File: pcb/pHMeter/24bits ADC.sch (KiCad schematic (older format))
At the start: 9 parts, among them J8 SJ, U6 HX711

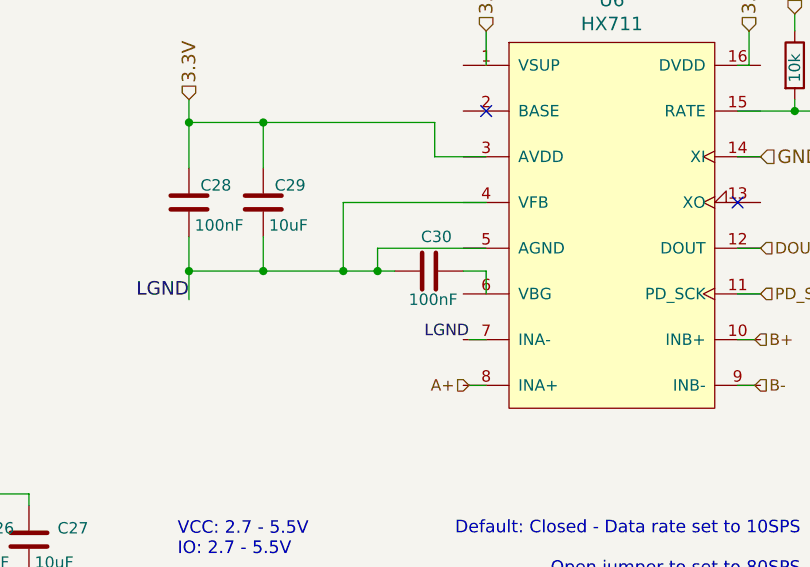
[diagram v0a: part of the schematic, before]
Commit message: Update pHMeter pcb
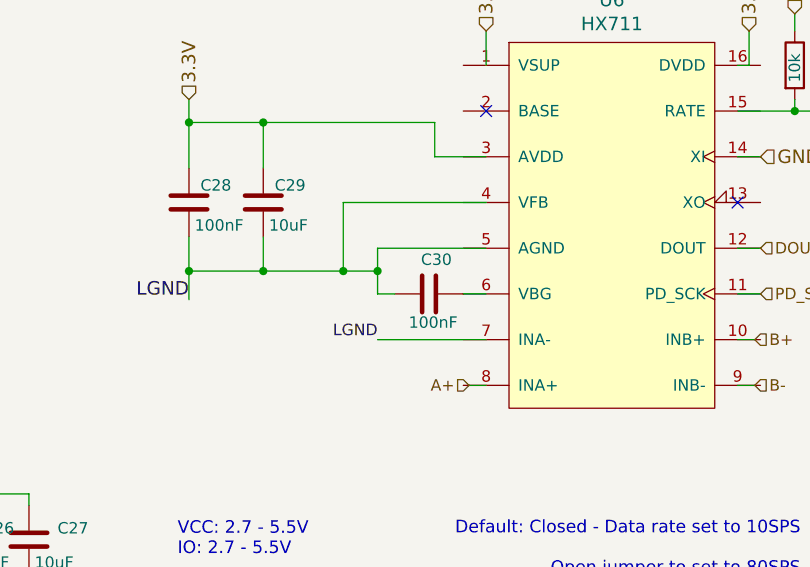
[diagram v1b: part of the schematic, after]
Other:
- moved on the sheet: C30
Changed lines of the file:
@@
 	3550 4600 3550 4700
-$Comp
-L Device:C C30
-U 1 1 5E3C27FC
-P 5875 3700
-F 0 "C30" V 6025 3600 50  0000 L CNN
-F 1 "100nF" V 5750 3575 50  0000 L CNN
-F 2 "Capacitor_SMD:C_0805_2012Metric_Pad1.15x1.40mm_HandSolder" H 5913 3550 50  0001 C CNN
-F 3 "~" H 5875 3700 50  0001 C CNN
-	1    5875 3700
-	0    -1   -1   0
-$EndComp
 $Comp
 L Device:C C28
@@
 	1    0    0    -1
 $EndComp
-Wire Wire Line
-	6025 3700 6125 3700
 Wire Wire Line
 	4825 3050 4825 3250
@@
 Wire Wire Line
 	5500 3400 5500 3700
-Connection ~ 5500 3700
-Wire Wire Line
-	5500 3700 5650 3700
-Wire Wire Line
-	5650 3600 5650 3700
 Connection ~ 5650 3700
 Wire Wire Line
-	5650 3700 5725 3700
-Wire Wire Line
 	7225 4200 7300 4200
-Wire Wire Line
-	6125 3700 6125 3800
 Wire Wire Line
 	5650 3600 6125 3600
@@
 	6125 2650 6125 2800
 Wire Wire Line
-	6050 4000 6125 4000
-Wire Wire Line
 	6050 4200 6125 4200
-Text Label 6050 4000 2    50   ~ 0
-LGND
 Text HLabel 6050 4200 0    50   Input ~ 0
 A+
@@
 	1    0    0    -1
 $EndComp
+Wire Wire Line
+	6025 3800 6125 3800
+Wire Wire Line
+	5650 3800 5725 3800
+$Comp
+L Device:C C30
+U 1 1 5E3C27FC
+P 5875 3800
+F 0 "C30" V 6025 3700 50  0000 L CNN
+F 1 "100nF" V 5750 3675 50  0000 L CNN
+F 2 "Capacitor_SMD:C_0805_2012Metric_Pad1.15x1.40mm_HandSolder" H 5913 3650 50  0001 C CNN
+F 3 "~" H 5875 3800 50  0001 C CNN
+	1    5875 3800
+	0    -1   -1   0
+$EndComp
+Wire Wire Line
+	5650 3700 5650 3800
+Connection ~ 5500 3700
+Wire Wire Line
+	5500 3700 5650 3700
+Wire Wire Line
+	5650 3600 5650 3700
+Text Label 5650 4000 2    50   ~ 0
+LGND
+Wire Wire Line
+	5650 4000 6125 4000
 $EndSCHEMATC
